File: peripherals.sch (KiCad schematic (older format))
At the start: 21 parts, among them J5 Micro_SD_Card_Det, J6 STRIP0, J7 STRIP1, J8 STRIP2, J9 STRIP3, SW2 BLE, SW3 CONFIG_RST, SW4 USER, U4 TXB0104D

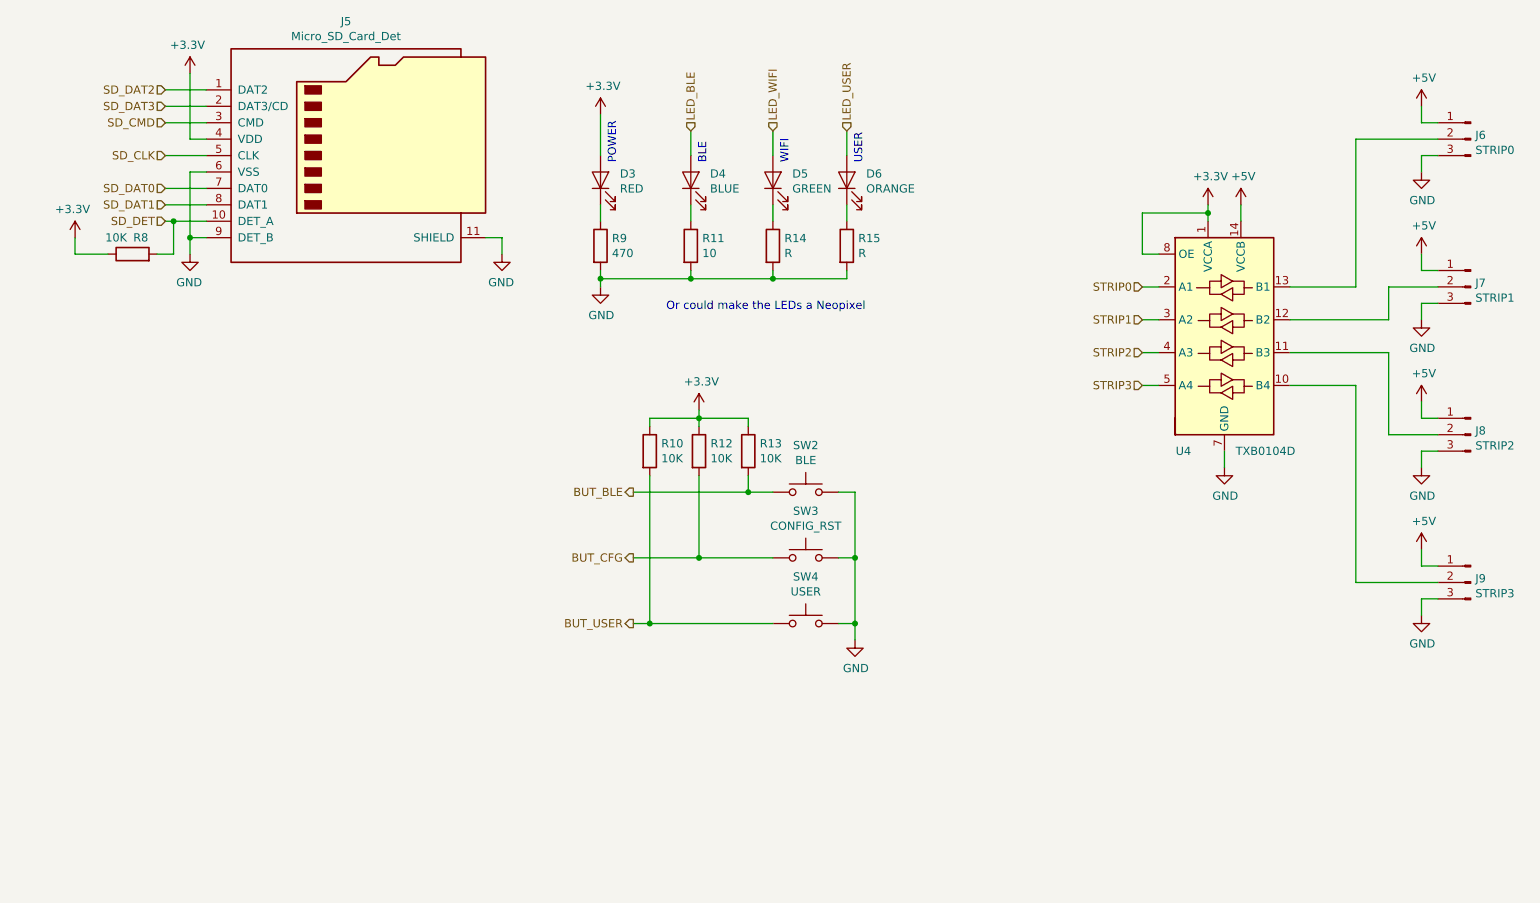
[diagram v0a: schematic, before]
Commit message: Ordered files
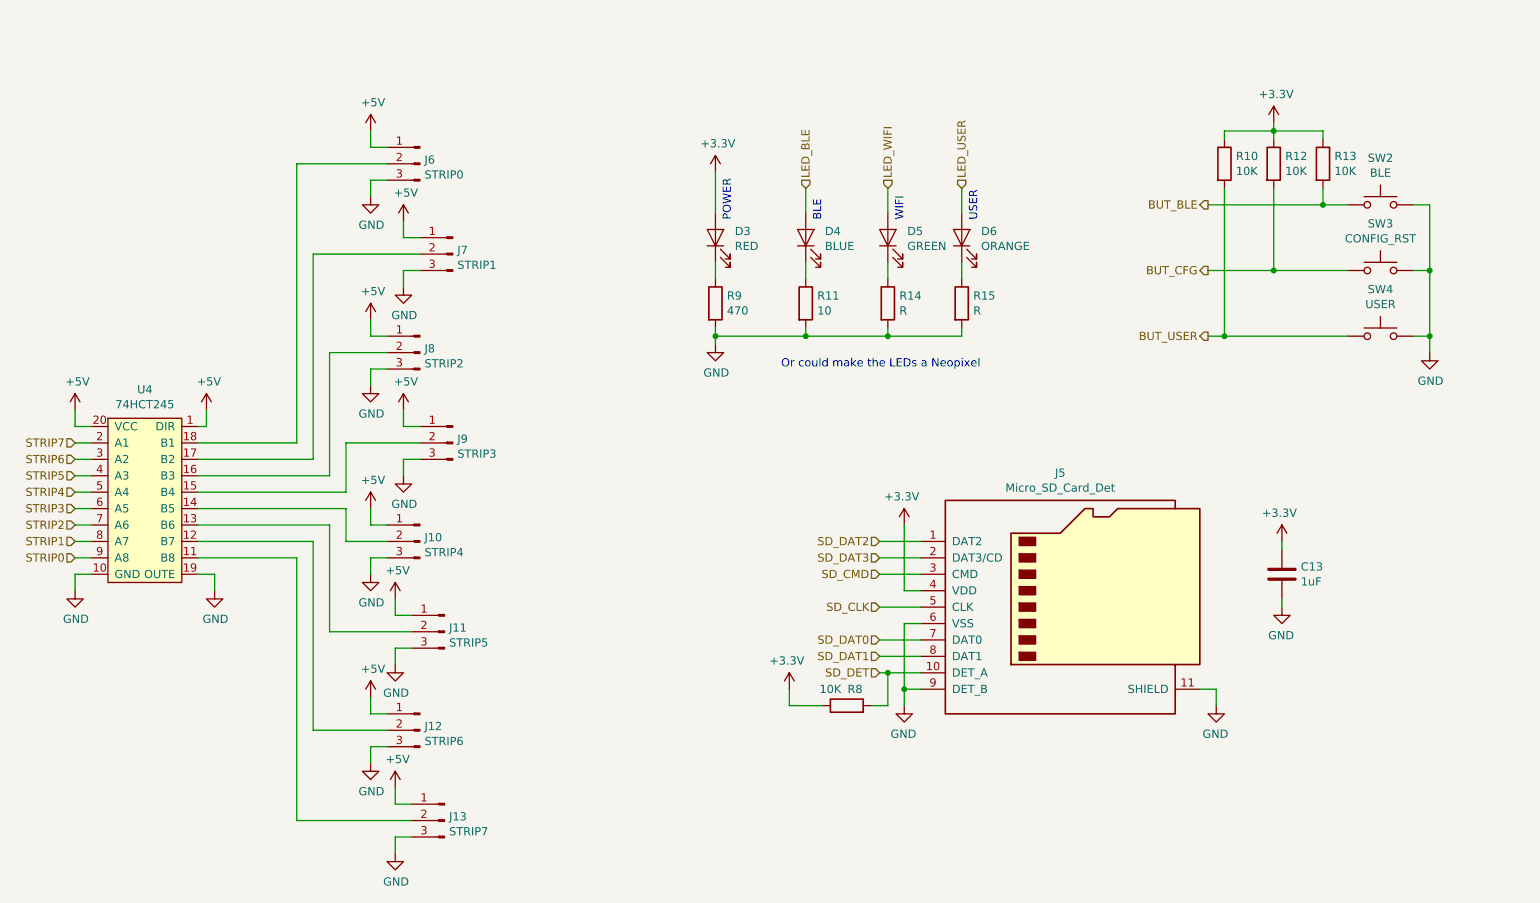
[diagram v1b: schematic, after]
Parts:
- removed U4: TXB0104D, Package_SO:SOIC-14_3.9x8.7mm_P1.27mm, symbol Logic_LevelTranslator:TXB0104D
- added C13: 1uF, Capacitor_SMD:C_0805_2012Metric, symbol Device:C
- added J10: STRIP4, Connector_PinHeader_2.54mm:PinHeader_1x03_P2.54mm_Vertical, symbol Connector:Conn_01x03_Male
- added J11: STRIP5, Connector_PinHeader_2.54mm:PinHeader_1x03_P2.54mm_Vertical, symbol Connector:Conn_01x03_Male
- added J12: STRIP6, Connector_PinHeader_2.54mm:PinHeader_1x03_P2.54mm_Vertical, symbol Connector:Conn_01x03_Male
- added J13: STRIP7, Connector_PinHeader_2.54mm:PinHeader_1x03_P2.54mm_Vertical, symbol Connector:Conn_01x03_Male
- added U4: 74HCT245, Package_SO:TSSOP-20_4.4x6.5mm_P0.65mm, symbol dot:74HCT245
- J5: footprint Connector_Card:microSD_HC_Hirose_DM3D-SF -> Connector_Card:microSD_HC_Hirose_DM3BT-DSF-PEJS
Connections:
- net +3V3: now also C13.1
- net +5V: now also J10.1 (Pin_1), J11.1 (Pin_1), J12.1 (Pin_1), J13.1 (Pin_1), U4.1 (DIR), U4.20 (VCC)
- net GND: now also C13.2, J10.3 (Pin_3), J11.3 (Pin_3), J12.3 (Pin_3), J13.3 (Pin_3), U4.10 (GND), U4.19 (OUTE)
- net STRIP0: now also U4.9 (A8)
- net STRIP1: now also U4.8 (A7)
- net STRIP2: now also U4.7 (A6)
- net STRIP3: now also U4.6 (A5)
- net at J6.2 (Pin_2): now also U4.18 (B1)
- net at J7.2 (Pin_2): now also U4.17 (B2)
- net at J8.2 (Pin_2): now also U4.16 (B3)
- net at J9.2 (Pin_2): now also U4.15 (B4)
- new net: J10.2 (Pin_2), U4.14 (B5)
- new net: J11.2 (Pin_2), U4.13 (B6)
- new net: J12.2 (Pin_2), U4.12 (B7)
- new net: J13.2 (Pin_2), U4.11 (B8)
- new net STRIP4: U4.5 (A4)
- new net STRIP5: U4.4 (A3)
- new net STRIP6: U4.3 (A2)
- new net STRIP7: U4.2 (A1)
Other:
- moved on the sheet: D3, D4, D5, D6, J5, J6, J7, J8, J9, R10, R11, R12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
